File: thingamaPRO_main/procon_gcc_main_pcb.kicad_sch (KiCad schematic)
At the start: 79 parts, among them J1 Rumble, J3 To Button Board, J4 Conn_01x06_Female, J5 Conn_01x02, J6 Conn_01x03_Male, J7 Rumble, J9 USB_C_Receptacle, Q1 Q_PMOS_GDS, Q2 Q_NMOS_GSD, Q3 Q_NMOS_GSD, SW1 SW_DIP_x04, SW3 SW_DIP_x01, U10 DRV5055A2xDBZxQ1, U11 DRV5055A2xDBZxQ1, U12 MCP3002, U13 PRTR5V0U2X, U14 XC6206PxxxMR, U15 RP2040, U2 2x DRV5053CAQLPGM Hall Effect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, U3 Stickbox_Assembly, U6 MCP3002, U7 DRV5055A2xDBZxQ1, U8 DRV5055A2xDBZxQ1, U9 W25Q128JVS, Y1 Crystal_GND3

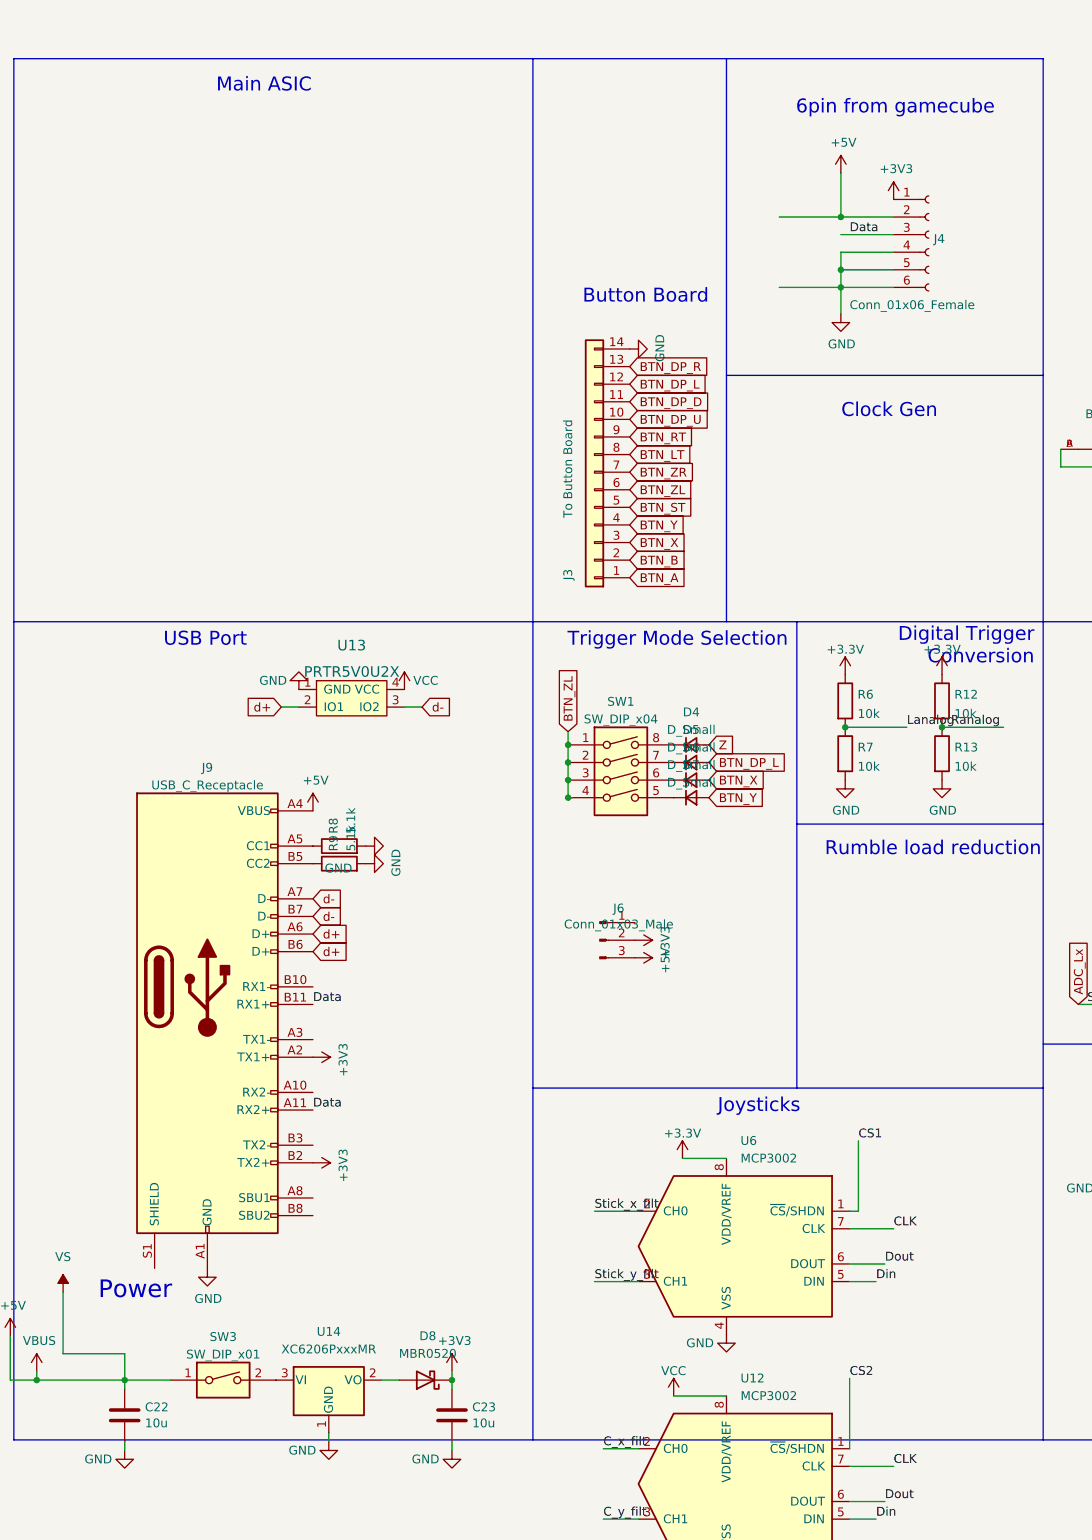
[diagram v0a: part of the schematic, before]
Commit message: Main pcb+bom shell/pos files
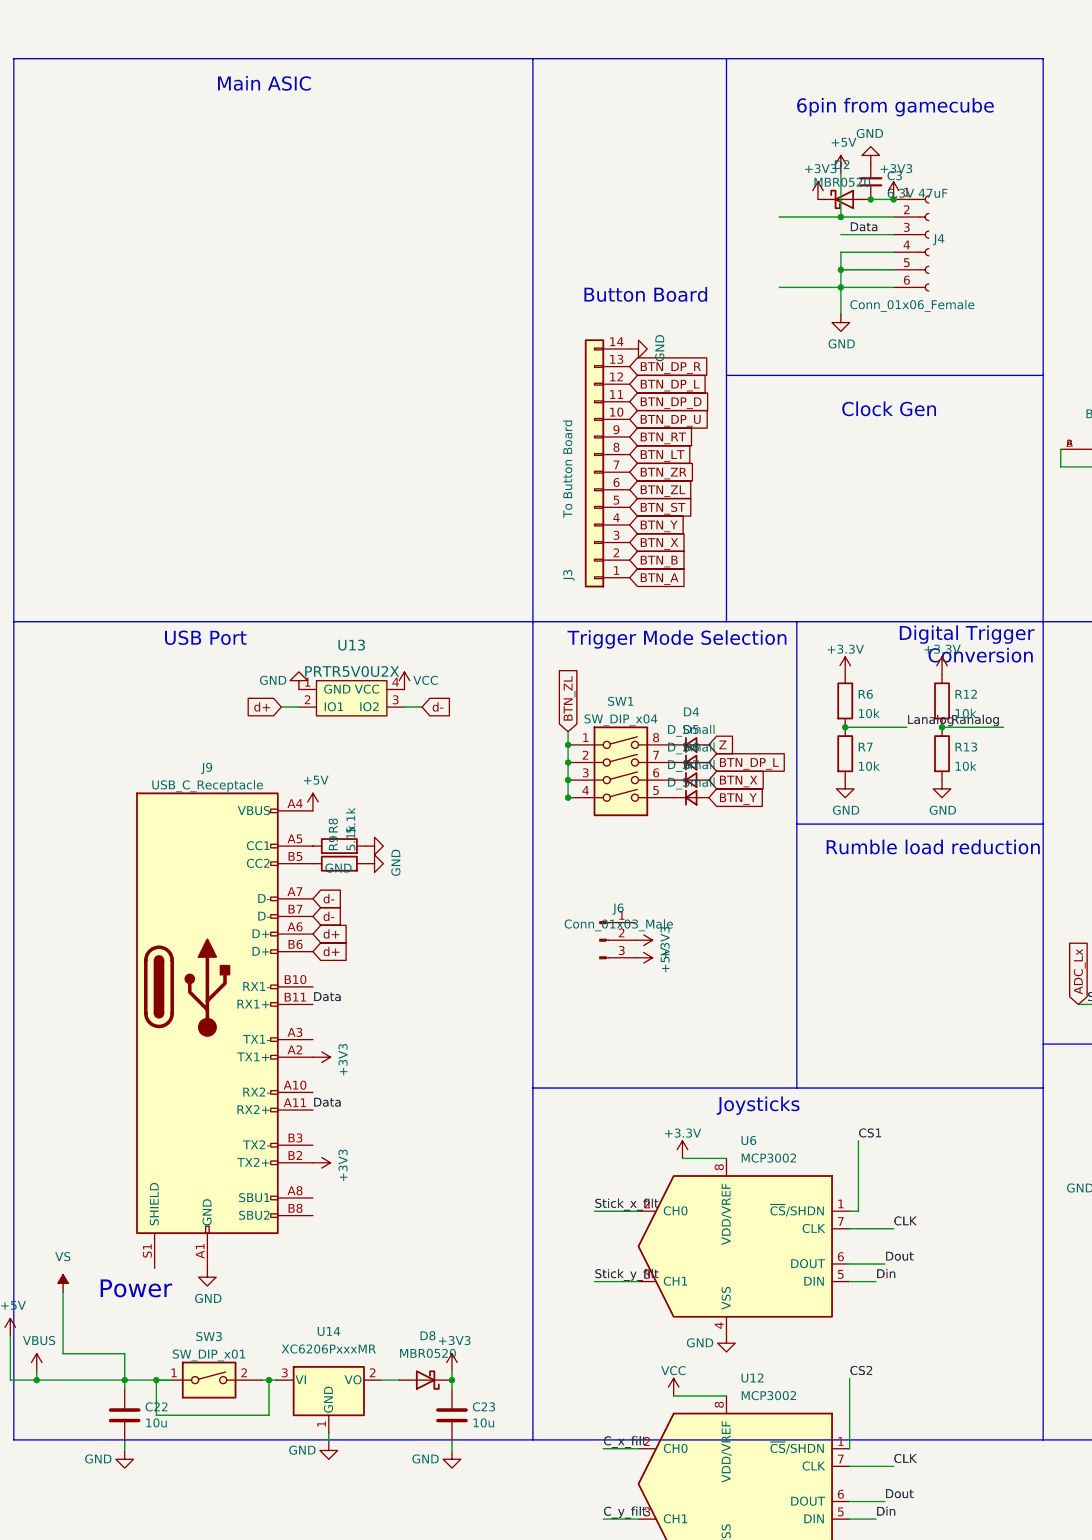
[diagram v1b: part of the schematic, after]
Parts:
- added C3: 6.3V 47uF, Capacitor_Tantalum_SMD:CP_EIA-3216-18_Kemet-A, symbol Device:C_Small
- added D2: MBR0520, Diode_SMD:D_SOD-323, symbol Diode:MBR0520
- D8: footprint PhobGCC_2_0_0_footprints:D_SOD-123 -> Diode_SMD:D_SOD-323
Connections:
- net +3V3: now also C3.1, D2.1 (K), D2.2 (A)
- net +5V: now also SW3.2, U14.3 (VI)
- net GND: now also C3.2
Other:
- moved on the sheet: SW3
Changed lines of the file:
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@@
     (company "Luberry's Custom Controllers")
   )
+  (junction (at 162.56 58.42) (diameter 0) (color 0 0 0 0)
+  )
   (junction (at 307.975 64.135) (diameter 0) (color 0 0 0 0)
   )
@@
   (junction (at 205.74 186.055) (diameter 0) (color 0 0 0 0)
   )
+  (junction (at 72.39 228.854) (diameter 0) (color 0 0 0 0)
+  )
   (junction (at 285.115 27.94) (diameter 0) (color 0 0 0 0)
   )
@@
   (junction (at 352.806 58.674) (diameter 0) (color 0 0 0 0)
   )
+  (junction (at 56.134 228.854) (diameter 0) (color 0 0 0 0)
+  )
   (junction (at 208.534 222.758) (diameter 0) (color 0 0 0 0)
   )
+  (junction (at 159.258 58.42) (diameter 0) (color 0 0 0 0)
+  )
   (junction (at 298.45 175.895) (diameter 0) (color 0 0 0 0)
   )
@@
     (stroke (width 0) (type default) (color 0 0 0 0))
   )
+  (wire (pts (xy 56.134 228.854) (xy 58.166 228.854))
+    (stroke (width 0) (type default) (color 0 0 0 0))
+  )
   (wire (pts (xy 132.08 196.85) (xy 138.43 196.85))
     (stroke (width 0) (type default) (color 0 0 0 0))
@@
     (stroke (width 0) (type default) (color 0 0 0 0))
   )
+  (wire (pts (xy 56.134 228.854) (xy 56.134 233.934))
+    (stroke (width 0) (type default) (color 0 0 0 0))
+  )
   (wire (pts (xy 371.602 124.46) (xy 374.142 124.46))
     (stroke (width 0) (type default) (color 0 0 0 0))
@@
     (stroke (width 0) (type default) (color 0 0 0 0))
   )
+  (wire (pts (xy 72.39 233.934) (xy 72.39 228.854))
+    (stroke (width 0) (type default) (color 0 0 0 0))
+  )
   (wire (pts (xy 368.808 29.845) (xy 368.935 29.845))
     (stroke (width 0) (type default) (color 0 0 0 0))
@@
     (stroke (width 0) (type default) (color 0 0 0 0))
   )
+  (wire (pts (xy 56.134 233.934) (xy 72.39 233.934))
+    (stroke (width 0) (type default) (color 0 0 0 0))
+  )
   (wire (pts (xy 347.472 124.46) (xy 344.932 124.46))
     (stroke (width 0) (type default) (color 0 0 0 0))
@@
     (stroke (width 0) (type default) (color 0 0 0 0))
   )
+  (wire (pts (xy 159.258 58.42) (xy 162.56 58.42))
+    (stroke (width 0) (type default) (color 0 0 0 0))
+  )
   (wire (pts (xy 411.48 37.084) (xy 411.48 62.484))
     (stroke (width 0) (type default) (color 0 0 0 0))
@@
     (stroke (width 0) (type default) (color 0 0 0 0))
   )
-  (wire (pts (xy 51.562 228.854) (xy 58.166 228.854))
+  (wire (pts (xy 51.562 228.854) (xy 56.134 228.854))
     (stroke (width 0) (type default) (color 0 0 0 0))
   )
@@
     (stroke (width 0) (type default) (color 0 0 0 0))
   )
+  (wire (pts (xy 71.374 228.854) (xy 72.39 228.854))
+    (stroke (width 0) (type default) (color 0 0 0 0))
+  )
   (wire (pts (xy 402.082 115.57) (xy 413.512 115.57))
     (stroke (width 0) (type default) (color 0 0 0 0))
   )
+  (wire (pts (xy 72.39 228.854) (xy 73.406 228.854))
+    (stroke (width 0) (type default) (color 0 0 0 0))
+  )
   (wire (pts (xy 285.115 44.45) (xy 257.175 44.45))
     (stroke (width 0) (type default) (color 0 0 0 0))
@@
     (pin "6")
   )
+  (symbol (lib_id "Device:C_Small") (at 159.258 55.88 180) (unit 1)
+    (in_bom yes) (on_board yes) (fields_autoplaced)
+    (property "Reference" "C3" (id 0) (at 161.5821 55.0389 0)
+      (effects (font (size 1.27 1.27)) (justify right))
+    )
+    (property "Value" "6.3V 47uF" (id 1) (at 161.5821 57.5758 0)
+      (effects (font (size 1.27 1.27)) (justify right))
+    )
+    (property "Footprint" "Capacitor_Tantalum_SMD:CP_EIA-3216-18_Kemet-A" (id 2) (at 159.258 55.88 0)
+      (effects (font (size 1.27 1.27)) hide)
+    )
+    (property "Datasheet" "~" (id 3) (at 159.258 55.88 0)
+      (effects (font (size 1.27 1.27)) hide)
+    )
+    (pin "1")
+    (pin "2")
+  )
   (symbol (lib_id "Sensor_Magnetic:DRV5055A2xDBZxQ1") (at 355.346 68.834 0) (unit 1)
     (in_bom yes) (on_board yes) (fields_autoplaced)
@@
     (pin "2")
   )
+  (symbol (lib_id "Diode:MBR0520") (at 155.448 58.42 0) (unit 1)
+    (in_bom yes) (on_board yes) (fields_autoplaced)
+    (property "Reference" "D2" (id 0) (at 155.1305 53.4502 0))
+    (property "Value" "MBR0520" (id 1) (at 155.1305 55.9871 0))
+    (property "Footprint" "Diode_SMD:D_SOD-323" (id 2) (at 155.448 62.865 0)
+      (effects (font (size 1.27 1.27)) hide)
+    )
+    (property "Datasheet" "http://www.mccsemi.com/up_pdf/MBR0520~MBR0580(SOD123).pdf" (id 3) (at 155.448 58.42 0)
+      (effects (font (size 1.27 1.27)) hide)
+    )
+    (pin "1")
+    (pin "2")
+  )
   (symbol (lib_id "power:GND") (at 63.5 212.725 0) (unit 1)
     (in_bom yes) (on_board yes)
@@
     (pin "2")
   )
-  (symbol (lib_id "Switch:SW_DIP_x01") (at 65.786 228.854 0) (unit 1)
+  (symbol (lib_id "Switch:SW_DIP_x01") (at 63.754 228.854 0) (unit 1)
     (in_bom yes) (on_board yes) (fields_autoplaced)
-    (property "Reference" "SW3" (id 0) (at 65.786 222.6142 0))
-    (property "Value" "SW_DIP_x01" (id 1) (at 65.786 225.1511 0))
-    (property "Footprint" "dips:switch_C381098" (id 2) (at 65.786 228.854 0)
+    (property "Reference" "SW3" (id 0) (at 63.754 222.6142 0))
+    (property "Value" "SW_DIP_x01" (id 1) (at 63.754 225.1511 0))
+    (property "Footprint" "dips:switch_C381098" (id 2) (at 63.754 228.854 0)
       (effects (font (size 1.27 1.27)) hide)
     )
-    (property "Datasheet" "~" (id 3) (at 65.786 228.854 0)
+    (property "Datasheet" "~" (id 3) (at 63.754 228.854 0)
       (effects (font (size 1.27 1.27)) hide)
     )
@@
     (pin "2")
   )
+  (symbol (lib_id "power:+3V3") (at 151.638 58.42 0) (unit 1)
+    (in_bom yes) (on_board yes)
+    (property "Reference" "#PWR0102" (id 0) (at 151.638 62.23 0)
+      (effects (font (size 1.27 1.27)) hide)
+    )
+    (property "Value" "+3V3" (id 1) (at 152.019 54.0258 0))
+    (property "Footprint" "" (id 2) (at 151.638 58.42 0)
+      (effects (font (size 1.27 1.27)) hide)
+    )
+    (property "Datasheet" "" (id 3) (at 151.638 58.42 0)
+      (effects (font (size 1.27 1.27)) hide)
+    )
+    (pin "1")
+  )
   (symbol (lib_id "power:GND") (at 86.36 154.305 90) (unit 1)
     (in_bom yes) (on_board yes)
@@
     (pin "1")
   )
+  (symbol (lib_id "power:GND") (at 159.258 53.34 180) (unit 1)
+    (in_bom yes) (on_board yes)
+    (property "Reference" "#PWR0101" (id 0) (at 159.258 46.99 0)
+      (effects (font (size 1.27 1.27)) hide)
+    )
+    (property "Value" "GND" (id 1) (at 159.131 48.9458 0))
+    (property "Footprint" "" (id 2) (at 159.258 53.34 0)
+      (effects (font (size 1.27 1.27)) hide)
+    )
+    (property "Datasheet" "" (id 3) (at 159.258 53.34 0)
+      (effects (font (size 1.27 1.27)) hide)
+    )
+    (pin "1")
+  )
   (symbol (lib_id "Device:R") (at 218.44 94.488 270) (unit 1)
     (in_bom yes) (on_board yes)
@@
     (property "Reference" "D8" (id 0) (at 95.3135 222.504 0))
     (property "Value" "MBR0520" (id 1) (at 95.3135 225.044 0))
-    (property "Footprint" "PhobGCC_2_0_0_footprints:D_SOD-123" (id 2) (at 94.996 224.409 0)
+    (property "Footprint" "Diode_SMD:D_SOD-323" (id 2) (at 94.996 224.409 0)
       (effects (font (size 1.27 1.27)) hide)
     )
@@
   )
   (symbol_instances
+    (path "/a94958c4-cb8d-4820-97f5-093934cfa737"
+      (reference "#PWR0101") (unit 1) (value "GND") (footprint "")
+    )
+    (path "/8a7623a3-4e0d-46b3-9b6f-61ae70c84f86"
+      (reference "#PWR0102") (unit 1) (value "+3V3") (footprint "")
+    )
     (path "/5e97ddfe-3d6f-4620-bfbb-4b22fefa11e6"
       (reference "#PWR0103") (unit 1) (value "GND") (footprint "")
@@
       (reference "C2") (unit 1) (value "1u") (footprint "Capacitor_SMD:C_0402_1005Metric")
     )
+    (path "/073eb6b3-b658-4280-b74a-7db6e352c115"
+      (reference "C3") (unit 1) (value "6.3V 47uF") (footprint "Capacitor_Tantalum_SMD:CP_EIA-3216-18_Kemet-A")
+    )
     (path "/d51f7905-dc84-4c6b-afdc-17f07fed6fc5"
       (reference "C9") (unit 1) (value "100n") (footprint "Capacitor_SMD:C_0402_1005Metric")
@@
       (reference "D1") (unit 1) (value "M7C") (footprint "PhobGCC_Footprints:D_SOD-123")
     )
+    (path "/4ea740f3-5246-4f88-aa0c-4a2a238987d1"
+      (reference "D2") (unit 1) (value "MBR0520") (footprint "Diode_SMD:D_SOD-323")
+    )
     (path "/b666148d-9905-4cc4-b448-65dd9dce4021"
       (reference "D4") (unit 1) (value "D_Small") (footprint "Diode_SMD:D_SOD-123")
@@
     )
     (path "/c51ee2df-daf8-4d13-b3ac-0b45d1a2356b"
-      (reference "D8") (unit 1) (value "MBR0520") (footprint "PhobGCC_2_0_0_footprints:D_SOD-123")
+      (reference "D8") (unit 1) (value "MBR0520") (footprint "Diode_SMD:D_SOD-323")
     )
     (path "/c6ac8fb4-80c7-4018-88c4-d054d9745114"
